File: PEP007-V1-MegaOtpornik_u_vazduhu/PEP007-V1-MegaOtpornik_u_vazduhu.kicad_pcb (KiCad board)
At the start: 2 copper layers, 45 x 45 mm, 9 parts, among them J1 Screw_Terminal_01x02

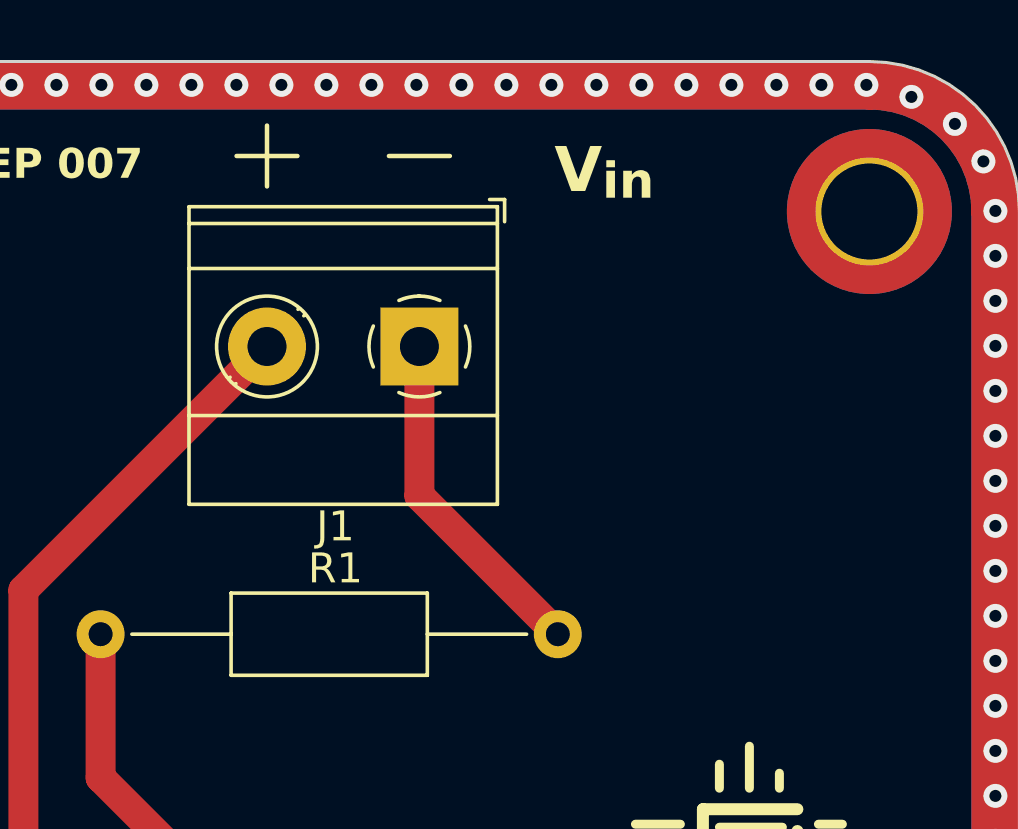
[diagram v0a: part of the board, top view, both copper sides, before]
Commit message: PEP007 and lib update.
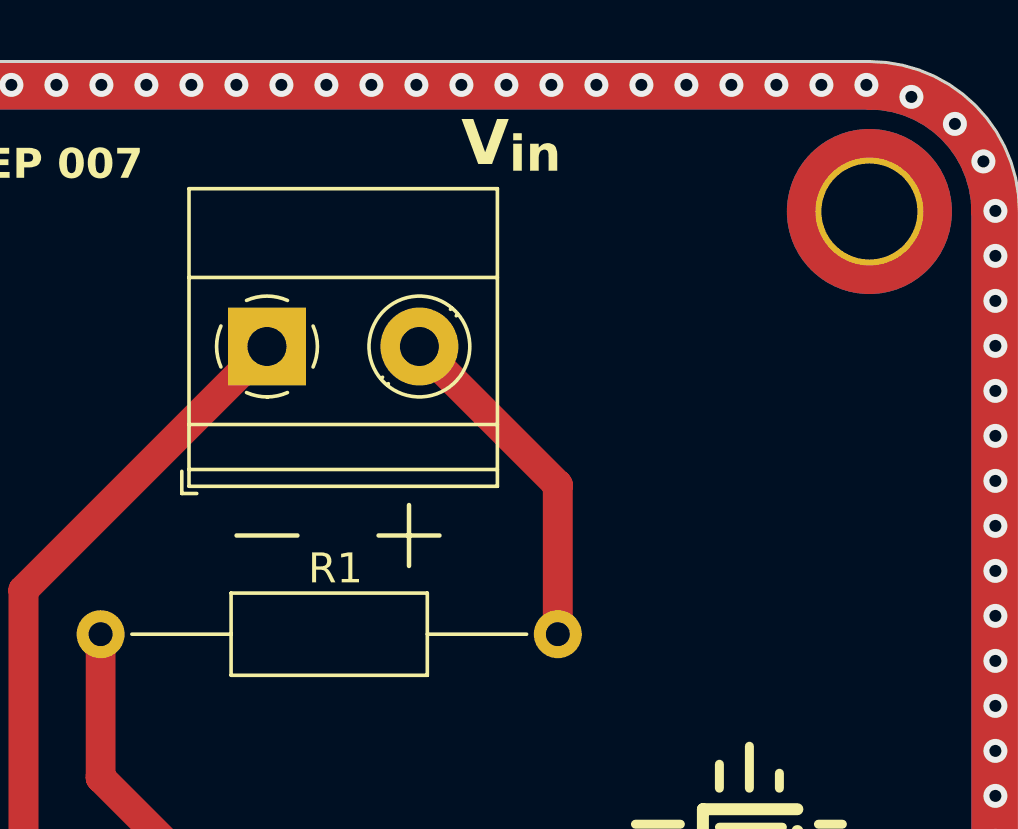
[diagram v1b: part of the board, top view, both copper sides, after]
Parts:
- removed J1: Screw_Terminal_01x02, PEP_library:TerminalBlock_Phoenix_MKDS-1,5-2-5.08_1x02_P5.08mm_Horizontal
- added J2: Klema, PEP_library:TerminalBlock_Phoenix_MKDS-1,5-2-5.08_1x02_P5.08mm_Horizontal, F.Cu at (119.9, 109.5)
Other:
- board text removed: "V_{in}"

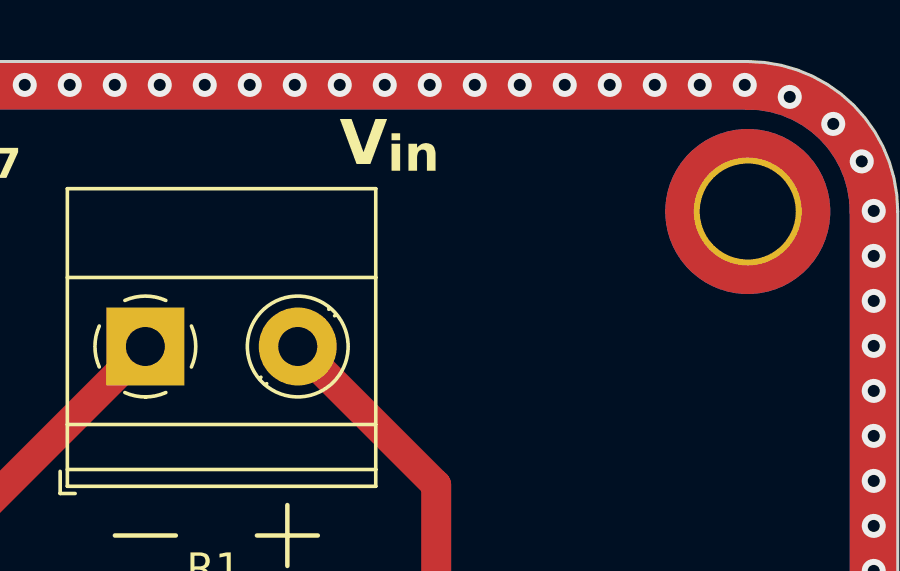
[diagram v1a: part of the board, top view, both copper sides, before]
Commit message: PEP007 final update, ready for production.
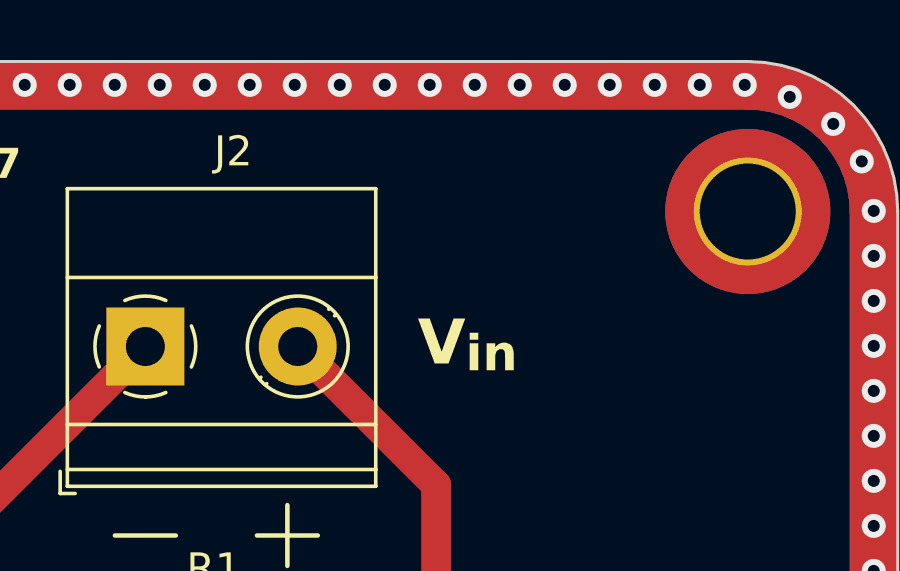
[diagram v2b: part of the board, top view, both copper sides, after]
